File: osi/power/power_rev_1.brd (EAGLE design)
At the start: 25.4 x 25.4 mm, 4 parts

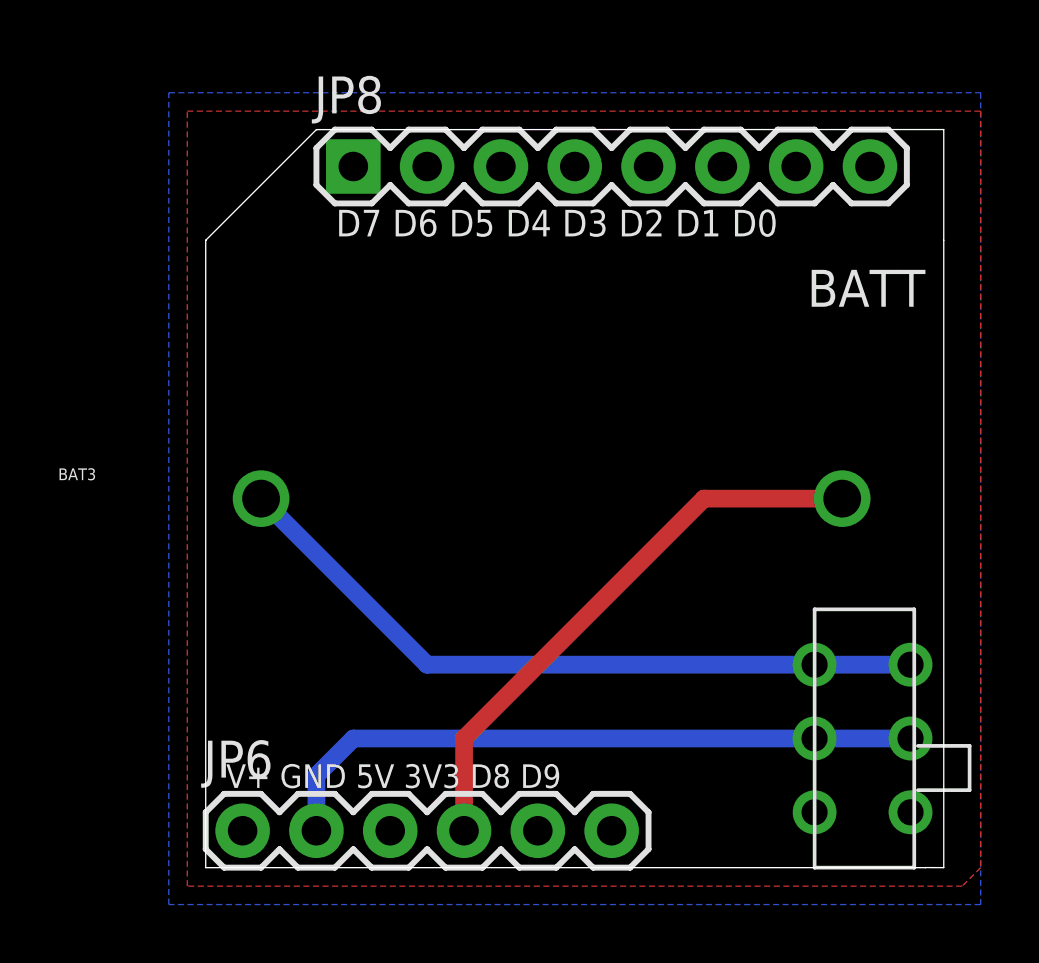
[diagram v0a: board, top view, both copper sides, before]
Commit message: update
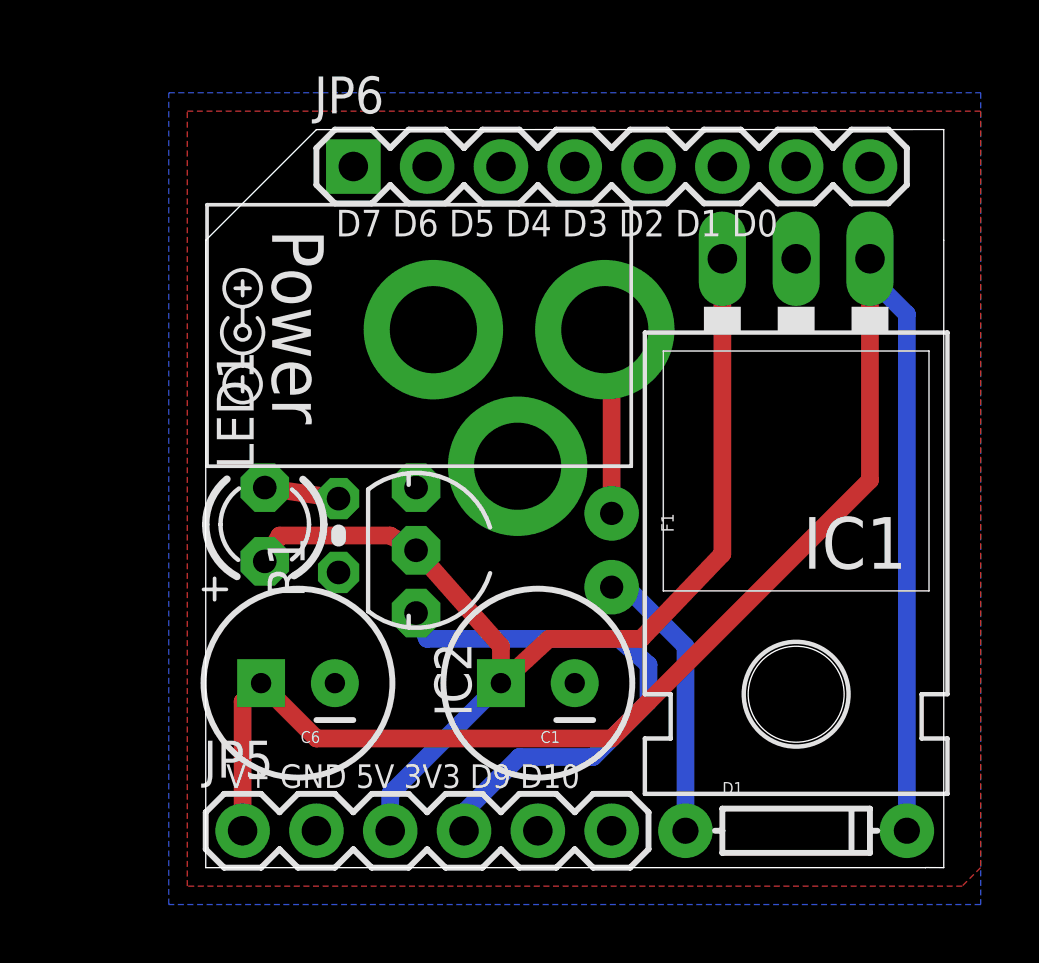
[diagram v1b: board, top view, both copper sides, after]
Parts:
- removed BAT3: (no value), SparkFun_mod:BATTCOM_20MM_PTH
- removed JP8: 8, SparkFun:1X08
- added C1, C6: (no value), SparkFun:CPOL-RADIAL-100UF-25V
- added D1: (no value), SparkFun:DIODE-1N4148
- added F1: PTCPTH, SparkFun_mod:PTC
- added IC1: (no value), SparkFun:TO-220-ALT
- added IC2: (no value), adafruit:TO92-INLINE
- added JP5: (no value), SparkFun:1X06
- added LED1: (no value), adafruit:LED3MM
- added R1: (no value), adafruit:0204V
- added U$2: (no value), DC_SYM:DC_POS_CTR
- added U$3: (no value), DC_SYM:DC_POS_CTR-BOTTOM
- JP6: value 6 -> (none); device SparkFun:1X06 -> SparkFun:1X08
- U$1: value SWITCH -> 2.1MMJACKTHM; device _my-parts:SWITCH -> adafruit:PJ-102A
- moved U$1 23.6 mm to (4.45, 18.4)
- moved JP6 23.2 mm to (5.08, 24.1)
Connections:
- removed net D8: JP6.5
- new net D10: JP5.6
- new net N$2: LED1.K, R1.2
- new net N$3: D1.A, F1.P$2
- net +3V3: now also IC2.3, JP5.4; no longer BAT3.1, JP6.4
- net +5V: now also C1.1, IC1.OUT, IC2.2, JP5.3, LED1.A; no longer JP6.3
- net AREF_D0: now also JP6.8; no longer JP8.8
- net D1: now also JP6.7; no longer JP8.7
- net D2: now also JP6.6; no longer JP8.6
- net D3: now also JP6.5; no longer JP8.5
- net D5: now also JP6.3; no longer JP8.3
- net D7: now also JP6.1; no longer JP8.1
- net D9: now also JP5.5; no longer JP6.6
- net GND: now also C1.2, C6.2, IC1.GND, IC2.1, JP5.2, R1.1, U$1.RING; no longer JP6.2, U$1.2, U$1.5
- net N$1: now also F1.P$1, U$1.TIP; no longer BAT3.2, U$1.3, U$1.6
- net SCL_D4: now also JP6.4; no longer JP8.4
- net SDA_D6: now also JP6.2; no longer JP8.2
- net V+: now also C6.1, D1.C, IC1.IN, JP5.1; no longer JP6.1
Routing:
- net V+: track 0.00 -> 59.2 mm
- net +5V: track 0.00 -> 37.8 mm
- net GND: track 22.9 -> 0.00 mm
- net N$1: track 24.7 -> 6.42 mm
- net N$3: track 0.00 -> 9.73 mm
- net N$2: track 0.00 -> 2.57 mm
- net +3V3: track 19.6 -> 18.8 mm
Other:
- board text added: "D10 D9 3V 5V GND V+"
- board text added: "Power"
- board text added: "Power Rev 1 Feb 12"
- board text added: "V+ GND 5V 3V3 D9 D10"
- board text removed: "BATT"
- board text removed: "Batt Rev 1 Feb 12"
- board text removed: "D8 D9 3V3 5V GND V+"
- board text removed: "V+ GND 5V 3V3 D8 D9"
